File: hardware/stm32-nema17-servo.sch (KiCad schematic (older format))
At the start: 90 parts, among them J1 Conn_01x05, J2 C31-S-RA-CS1A-BK-SS, J3 TC-2050, J4 Screw_Terminal_01x02, J5 Screw_Terminal_01x02, J7 Conn_01x03, J8 Conn_01x03, J9 Conn_01x02, M1 Stepper_Motor_bipolar, Q1 NTTFS4937N, Q10 SSM3K35CTC, Q2 NVTFS5C658NL, Q3 NVTFS5C658NL, Q4 NVTFS5C658NL, Q5 NVTFS5C658NL, Q6 NVTFS5C658NL, Q7 NVTFS5C658NL, Q8 SSM3K35CTC, Q9 SSM3K35CTC, SW1 EVP-BB2A9B000, U1 STM32G431CBU, U3 UCC27516, U4 AS5047D, U5 TPS62172DSG, U6 DRV8323RS

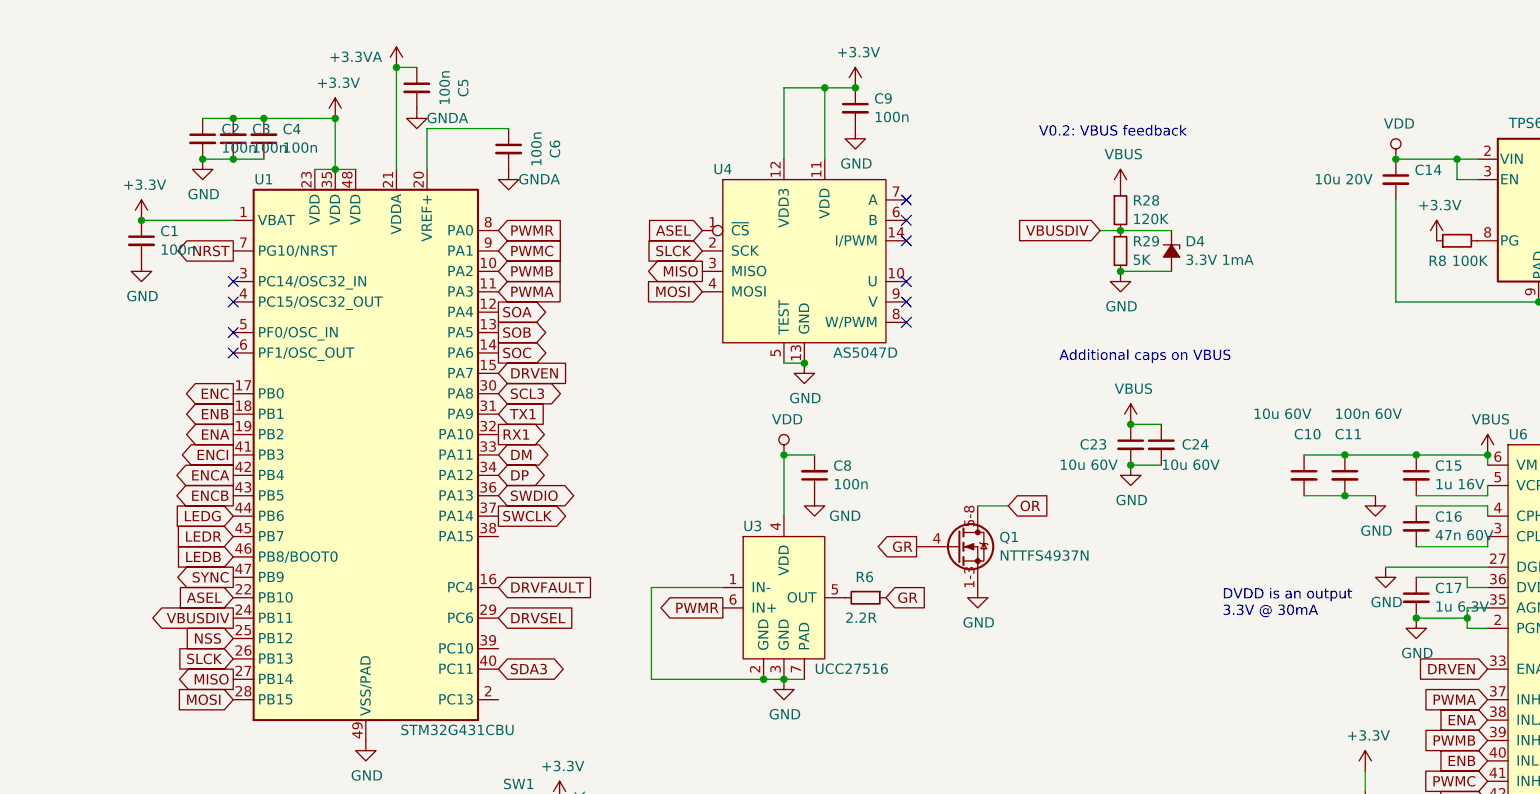
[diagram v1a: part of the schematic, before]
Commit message: hardware version 0.2 as sent to board fab
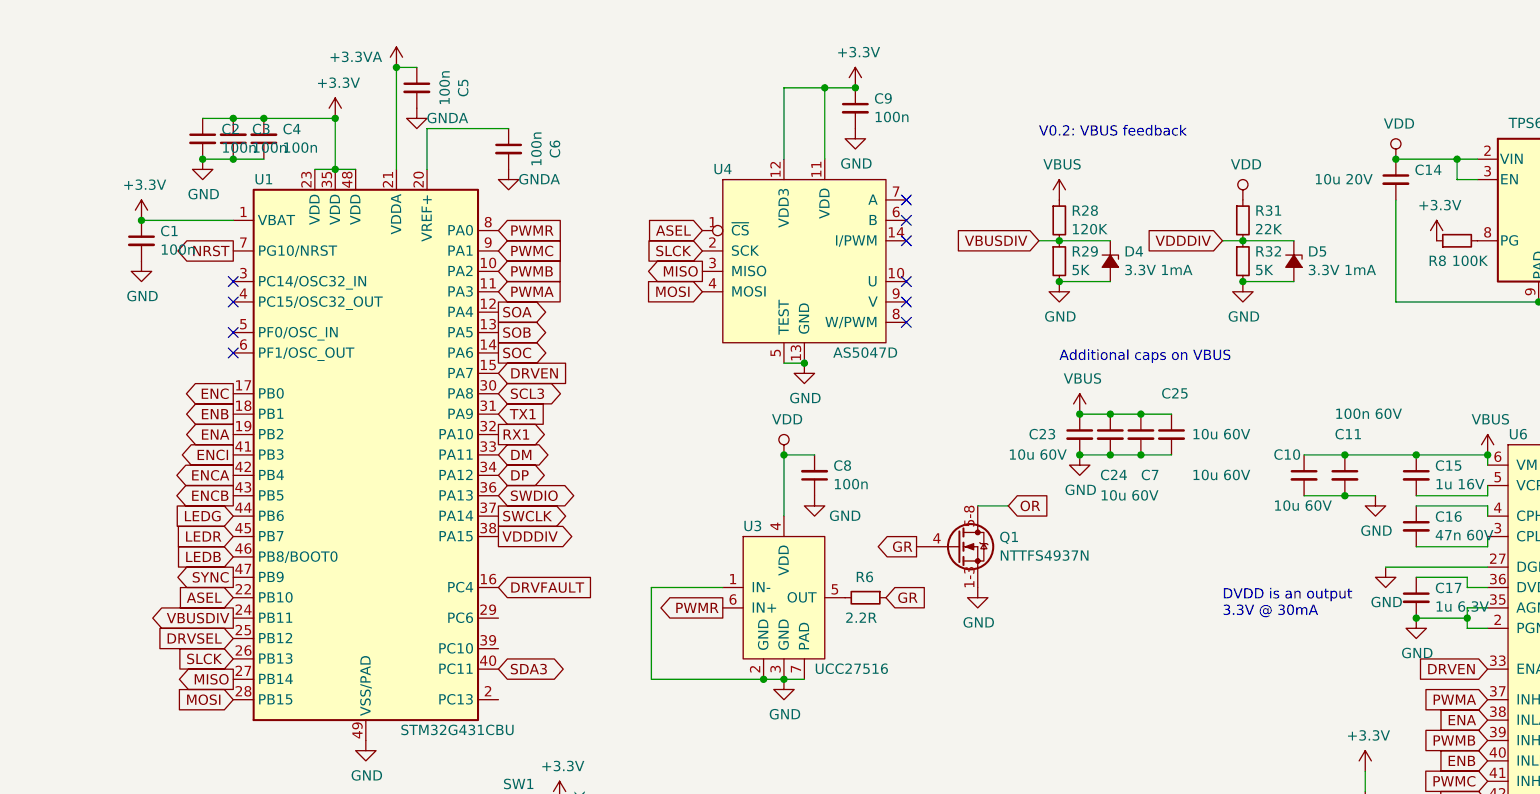
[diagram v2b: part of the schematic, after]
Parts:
- added C25, C7: 10u 60V, Capacitor_SMD:C_1210_3225Metric, symbol Device:C_Small
- added D5: 3.3V 1mA, Diode_SMD:D_0402_1005Metric, symbol Device:D_Zener_Small_ALT
- added R31: 22K, Resistor_SMD:R_0402_1005Metric, symbol Device:R_Small
- added R32: 5K, Resistor_SMD:R_0402_1005Metric, symbol Device:R_Small
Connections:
- net NSS is gone; now on net DRVSEL: U1.25 (PB12)
- net DRVSEL: no longer U1.29 (PC6)
- net GND: now also C25.2, C7.2, D5.2 (A), R32.2
- net VBUS: now also C25.1, C7.1
- net VDD: now also R31.1
- net VDDDIV: now reaches U1.38 (PA15)
- net VDDDIV: now also D5.1 (K), R31.2, R32.1
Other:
- moved on the sheet: C23, C24, D4, R28, R29
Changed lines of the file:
@@
-EESchema Schematic File Version 5
+EESchema Schematic File Version 4
 LIBS:stm32-nema17-servo-cache
 EELAYER 30 0
@@
 U 1 1 5D4F5968
 P 6550 2800
-F 0 "C10" H 6500 3000 50  0000 L CNN
-F 1 "10u 60V" H 6300 3100 50  0000 L CNN
+F 0 "C10" H 6400 2900 50  0000 L CNN
+F 1 "10u 60V" H 6400 2650 50  0000 L CNN
 F 2 "Capacitor_SMD:C_1210_3225Metric" H 6550 2800 50  0001 C CNN
 F 3 "~" H 6550 2800 50  0001 C CNN
@@
 Text GLabel 10400 1300 0    50   Output ~ 0
 OB
-Text GLabel 1300 3600 0    50   Input ~ 0
-NSS
 Text Notes 7850 2300 0    50   ~ 0
 DRV8323 cannot be daisy-chained on SPI
@@
 	3150 6300 3550 6300
 Connection ~ 3150 6300
-Text GLabel 2600 3500 2    50   Input ~ 0
+Text GLabel 1300 3600 0    50   Input ~ 0
 DRVSEL
 Text GLabel 1300 3400 0    50   Input ~ 0
@@
 L Device:C_Small C23
 U 1 1 5D56448D
-P 5700 2650
-F 0 "C23" H 5450 2650 50  0000 L CNN
-F 1 "10u 60V" H 5350 2550 50  0000 L CNN
-F 2 "Capacitor_SMD:C_1210_3225Metric" H 5700 2650 50  0001 C CNN
-F 3 "~" H 5700 2650 50  0001 C CNN
-	1    5700 2650
+P 5450 2600
+F 0 "C23" H 5200 2600 50  0000 L CNN
+F 1 "10u 60V" H 5100 2500 50  0000 L CNN
+F 2 "Capacitor_SMD:C_1210_3225Metric" H 5450 2600 50  0001 C CNN
+F 3 "~" H 5450 2600 50  0001 C CNN
+	1    5450 2600
 	1    0    0    -1
 $EndComp
@@
 L power:VBUS #PWR059
 U 1 1 5D567754
-P 5700 2550
-F 0 "#PWR059" H 5700 2400 50  0001 C CNN
-F 1 "VBUS" H 5715 2723 50  0000 C CNN
-F 2 "" H 5700 2550 50  0001 C CNN
-F 3 "" H 5700 2550 50  0001 C CNN
-	1    5700 2550
+P 5450 2500
+F 0 "#PWR059" H 5450 2350 50  0001 C CNN
+F 1 "VBUS" H 5465 2673 50  0000 C CNN
+F 2 "" H 5450 2500 50  0001 C CNN
+F 3 "" H 5450 2500 50  0001 C CNN
+	1    5450 2500
 	1    0    0    -1
 $EndComp
@@
 L power:GND #PWR060
 U 1 1 5D56F0C9
-P 5700 2750
-F 0 "#PWR060" H 5700 2500 50  0001 C CNN
-F 1 "GND" H 5705 2577 50  0000 C CNN
-F 2 "" H 5700 2750 50  0001 C CNN
-F 3 "" H 5700 2750 50  0001 C CNN
-	1    5700 2750
+P 5450 2700
+F 0 "#PWR060" H 5450 2450 50  0001 C CNN
+F 1 "GND" H 5455 2527 50  0000 C CNN
+F 2 "" H 5450 2700 50  0001 C CNN
+F 3 "" H 5450 2700 50  0001 C CNN
+	1    5450 2700
 	1    0    0    -1
 $EndComp
@@
 L Device:C_Small C24
 U 1 1 5D57E91C
-P 5850 2650
-F 0 "C24" H 5950 2650 50  0000 L CNN
-F 1 "10u 60V" H 5850 2550 50  0000 L CNN
-F 2 "Capacitor_SMD:C_1210_3225Metric" H 5850 2650 50  0001 C CNN
-F 3 "~" H 5850 2650 50  0001 C CNN
-	1    5850 2650
-	1    0    0    -1
-$EndComp
-Wire Wire Line
-	5700 2550 5850 2550
-Connection ~ 5700 2550
-Wire Wire Line
-	5850 2750 5700 2750
-Connection ~ 5700 2750
+P 5600 2600
+F 0 "C24" H 5550 2400 50  0000 L CNN
+F 1 "10u 60V" H 5550 2300 50  0000 L CNN
+F 2 "Capacitor_SMD:C_1210_3225Metric" H 5600 2600 50  0001 C CNN
+F 3 "~" H 5600 2600 50  0001 C CNN
+	1    5600 2600
+	1    0    0    -1
+$EndComp
+Wire Wire Line
+	5450 2500 5600 2500
+Connection ~ 5450 2500
+Wire Wire Line
+	5600 2700 5450 2700
+Connection ~ 5450 2700
 $Comp
 L Switch:SW_Push SW1
@@
 L Device:R_Small R28
 U 1 1 5D668B4B
-P 5650 1500
-F 0 "R28" H 5709 1546 50  0000 L CNN
-F 1 "120K" H 5709 1455 50  0000 L CNN
-F 2 "Resistor_SMD:R_0402_1005Metric" H 5650 1500 50  0001 C CNN
-F 3 "~" H 5650 1500 50  0001 C CNN
-	1    5650 1500
+P 5350 1550
+F 0 "R28" H 5409 1596 50  0000 L CNN
+F 1 "120K" H 5409 1505 50  0000 L CNN
+F 2 "Resistor_SMD:R_0402_1005Metric" H 5350 1550 50  0001 C CNN
+F 3 "~" H 5350 1550 50  0001 C CNN
+	1    5350 1550
 	1    0    0    -1
 $EndComp
@@
 L Device:R_Small R29
 U 1 1 5D668B59
-P 5650 1700
-F 0 "R29" H 5709 1746 50  0000 L CNN
-F 1 "5K" H 5709 1655 50  0000 L CNN
-F 2 "Resistor_SMD:R_0402_1005Metric" H 5650 1700 50  0001 C CNN
-F 3 "~" H 5650 1700 50  0001 C CNN
-	1    5650 1700
+P 5350 1750
+F 0 "R29" H 5409 1796 50  0000 L CNN
+F 1 "5K" H 5409 1705 50  0000 L CNN
+F 2 "Resistor_SMD:R_0402_1005Metric" H 5350 1750 50  0001 C CNN
+F 3 "~" H 5350 1750 50  0001 C CNN
+	1    5350 1750
 	1    0    0    -1
 $EndComp
@@
 L power:VBUS #PWR063
 U 1 1 5D66DC6D
-P 5650 1400
-F 0 "#PWR063" H 5650 1250 50  0001 C CNN
-F 1 "VBUS" H 5665 1573 50  0000 C CNN
-F 2 "" H 5650 1400 50  0001 C CNN
-F 3 "" H 5650 1400 50  0001 C CNN
-	1    5650 1400
+P 5350 1450
+F 0 "#PWR063" H 5350 1300 50  0001 C CNN
+F 1 "VBUS" H 5365 1623 50  0000 C CNN
+F 2 "" H 5350 1450 50  0001 C CNN
+F 3 "" H 5350 1450 50  0001 C CNN
+	1    5350 1450
 	1    0    0    -1
 $EndComp
@@
 L Device:D_Zener_Small_ALT D4
 U 1 1 5D67431D
-P 5900 1700
-F 0 "D4" V 5854 1768 50  0000 L CNN
-F 1 "3.3V 1mA" V 5945 1768 50  0000 L CNN
-F 2 "Diode_SMD:D_0402_1005Metric" V 5900 1700 50  0001 C CNN
-F 3 "~" V 5900 1700 50  0001 C CNN
-	1    5900 1700
+P 5600 1750
+F 0 "D4" V 5554 1818 50  0000 L CNN
+F 1 "3.3V 1mA" V 5645 1818 50  0000 L CNN
+F 2 "Diode_SMD:D_0402_1005Metric" V 5600 1750 50  0001 C CNN
+F 3 "~" V 5600 1750 50  0001 C CNN
+	1    5600 1750
 	0    1    1    0
 $EndComp
@@
 L power:GND #PWR064
 U 1 1 5D679087
-P 5650 1800
-F 0 "#PWR064" H 5650 1550 50  0001 C CNN
-F 1 "GND" H 5655 1627 50  0000 C CNN
-F 2 "" H 5650 1800 50  0001 C CNN
-F 3 "" H 5650 1800 50  0001 C CNN
-	1    5650 1800
-	1    0    0    -1
-$EndComp
-Wire Wire Line
-	5650 1800 5900 1800
-Connection ~ 5650 1800
-Wire Wire Line
-	5900 1600 5650 1600
-Connection ~ 5650 1600
-Text GLabel 5550 1600 0    50   Input ~ 0
+P 5350 1850
+F 0 "#PWR064" H 5350 1600 50  0001 C CNN
+F 1 "GND" H 5355 1677 50  0000 C CNN
+F 2 "" H 5350 1850 50  0001 C CNN
+F 3 "" H 5350 1850 50  0001 C CNN
+	1    5350 1850
+	1    0    0    -1
+$EndComp
+Wire Wire Line
+	5350 1850 5600 1850
+Connection ~ 5350 1850
+Wire Wire Line
+	5600 1650 5350 1650
+Connection ~ 5350 1650
+Text GLabel 5250 1650 0    50   Input ~ 0
 VBUSDIV
 Wire Wire Line
-	5550 1600 5650 1600
+	5250 1650 5350 1650
 Text Notes 5250 1150 0    50   ~ 0
 V0.2: VBUS feedback
@@
 Wire Wire Line
 	6850 4650 7450 4650
+$Comp
+L Device:C_Small C7
+U 1 1 5DA4E6B2
+P 5750 2600
+F 0 "C7" H 5750 2400 50  0000 L CNN
+F 1 "10u 60V" H 6000 2400 50  0000 L CNN
+F 2 "Capacitor_SMD:C_1210_3225Metric" H 5750 2600 50  0001 C CNN
+F 3 "~" H 5750 2600 50  0001 C CNN
+	1    5750 2600
+	1    0    0    -1
+$EndComp
+Wire Wire Line
+	5600 2500 5750 2500
+Connection ~ 5600 2500
+Wire Wire Line
+	5600 2700 5750 2700
+Connection ~ 5600 2700
+Text GLabel 2600 3100 2    50   Output ~ 0
+VDDDIV
+$Comp
+L Device:R_Small R31
+U 1 1 5DB3AAC1
+P 6250 1550
+F 0 "R31" H 6309 1596 50  0000 L CNN
+F 1 "22K" H 6309 1505 50  0000 L CNN
+F 2 "Resistor_SMD:R_0402_1005Metric" H 6250 1550 50  0001 C CNN
+F 3 "~" H 6250 1550 50  0001 C CNN
+	1    6250 1550
+	1    0    0    -1
+$EndComp
+$Comp
+L Device:R_Small R32
+U 1 1 5DB3AACB
+P 6250 1750
+F 0 "R32" H 6309 1796 50  0000 L CNN
+F 1 "5K" H 6309 1705 50  0000 L CNN
+F 2 "Resistor_SMD:R_0402_1005Metric" H 6250 1750 50  0001 C CNN
+F 3 "~" H 6250 1750 50  0001 C CNN
+	1    6250 1750
+	1    0    0    -1
+$EndComp
+$Comp
+L Device:D_Zener_Small_ALT D5
+U 1 1 5DB3AADF
+P 6500 1750
+F 0 "D5" V 6454 1818 50  0000 L CNN
+F 1 "3.3V 1mA" V 6545 1818 50  0000 L CNN
+F 2 "Diode_SMD:D_0402_1005Metric" V 6500 1750 50  0001 C CNN
+F 3 "~" V 6500 1750 50  0001 C CNN
+	1    6500 1750
+	0    1    1    0
+$EndComp
+$Comp
+L power:GND #PWR018
+U 1 1 5DB3AAE9
+P 6250 1850
+F 0 "#PWR018" H 6250 1600 50  0001 C CNN
+F 1 "GND" H 6255 1677 50  0000 C CNN
+F 2 "" H 6250 1850 50  0001 C CNN
+F 3 "" H 6250 1850 50  0001 C CNN
+	1    6250 1850
+	1    0    0    -1
+$EndComp
+Wire Wire Line
+	6250 1850 6500 1850
+Connection ~ 6250 1850
+Wire Wire Line
+	6500 1650 6250 1650
+Connection ~ 6250 1650
+Text GLabel 6150 1650 0    50   Input ~ 0
+VDDDIV
+Wire Wire Line
+	6150 1650 6250 1650
+$Comp
+L power:VDD #PWR0110
+U 1 1 5DB71341
+P 6250 1450
+F 0 "#PWR0110" H 6250 1300 50  0001 C CNN
+F 1 "VDD" H 6267 1623 50  0000 C CNN
+F 2 "" H 6250 1450 50  0001 C CNN
+F 3 "" H 6250 1450 50  0001 C CNN
+	1    6250 1450
+	1    0    0    -1
+$EndComp
+$Comp
+L Device:C_Small C25
+U 1 1 5DE23E59
+P 5900 2600
+F 0 "C25" H 5850 2800 50  0000 L CNN
+F 1 "10u 60V" H 6000 2600 50  0000 L CNN
+F 2 "Capacitor_SMD:C_1210_3225Metric" H 5900 2600 50  0001 C CNN
+F 3 "~" H 5900 2600 50  0001 C CNN
+	1    5900 2600
+	1    0    0    -1
+$EndComp
+Wire Wire Line
+	5750 2500 5900 2500
+Connection ~ 5750 2500
+Wire Wire Line
+	5750 2700 5900 2700
+Connection ~ 5750 2700
 $EndSCHEMATC
